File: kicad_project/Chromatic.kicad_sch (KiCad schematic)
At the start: 159 parts, among them J1 J1, J2 J2

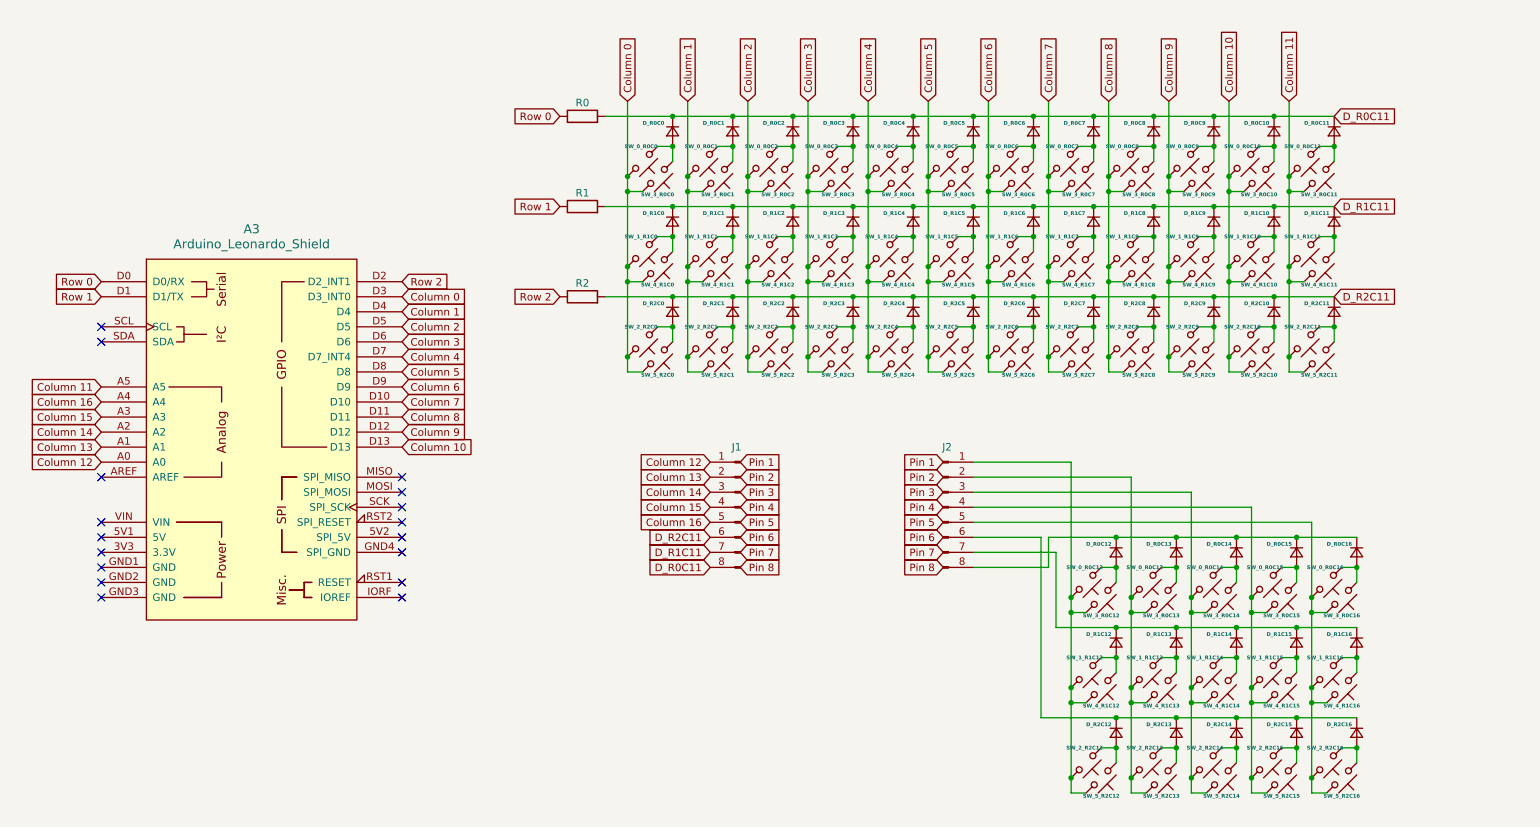
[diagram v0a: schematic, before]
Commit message: done
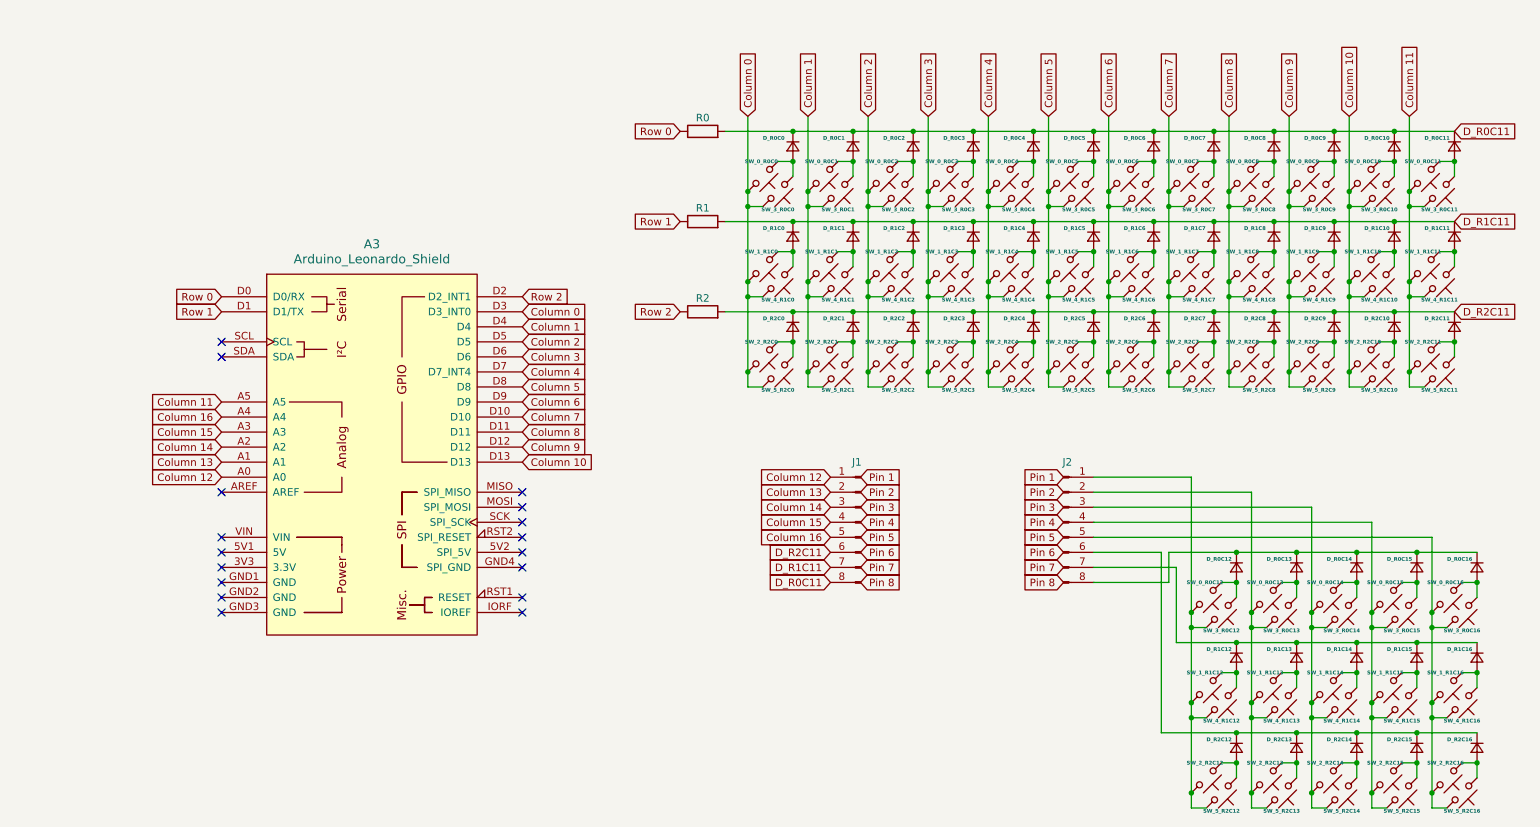
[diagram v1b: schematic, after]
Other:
- moved on the sheet: A3, D_R0C0, D_R0C1, D_R0C10, D_R0C11, D_R0C12, D_R0C13, D_R0C14, D_R0C15, D_R0C16, D_R0C2, D_R0C3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
